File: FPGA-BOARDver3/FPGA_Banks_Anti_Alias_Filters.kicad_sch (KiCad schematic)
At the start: 10 parts, among them U1 XC7Z020-1CLG400I__

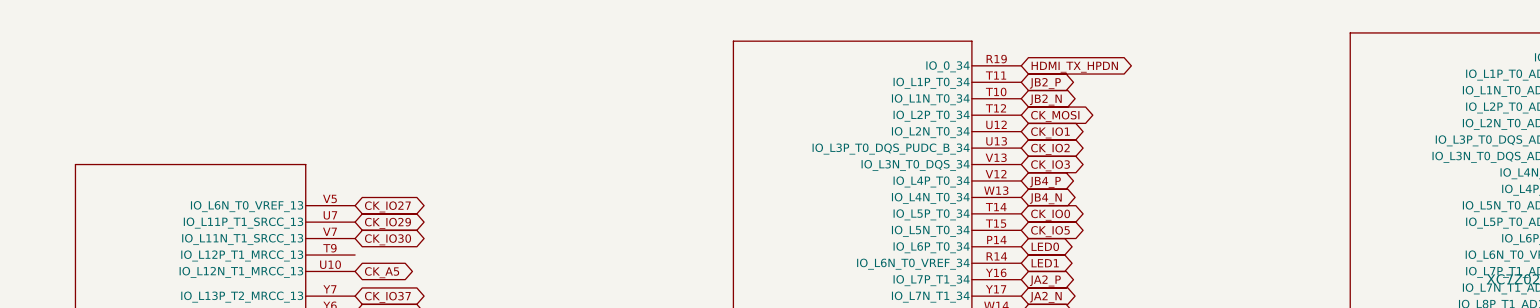
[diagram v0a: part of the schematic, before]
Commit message: update
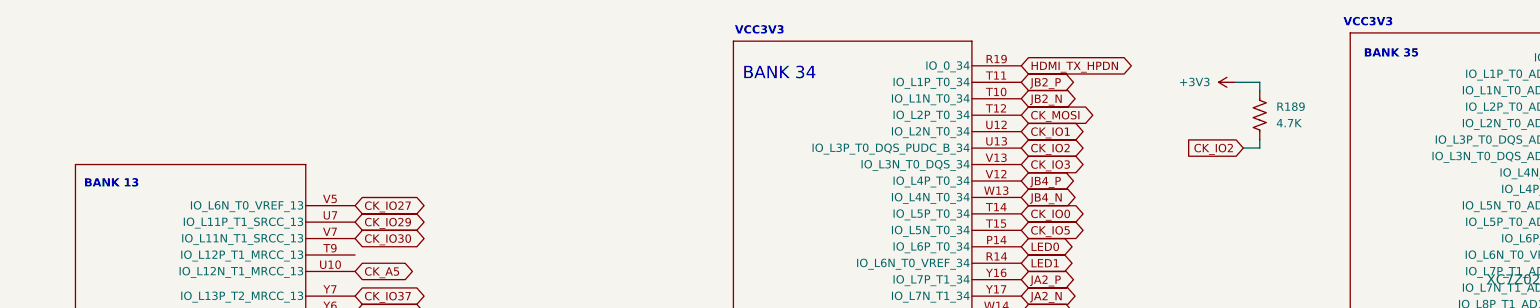
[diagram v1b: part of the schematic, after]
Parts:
- added R189: 4.7K, footprints:R_0402, symbol Device:R_US
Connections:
- net CK_IO2: now also R189.1
- new net +3V3: R189.2
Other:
- note added: "BANK 13"
- note added: "BANK 34"
- note added: "BANK 35"
- note added: "VCC3V3"

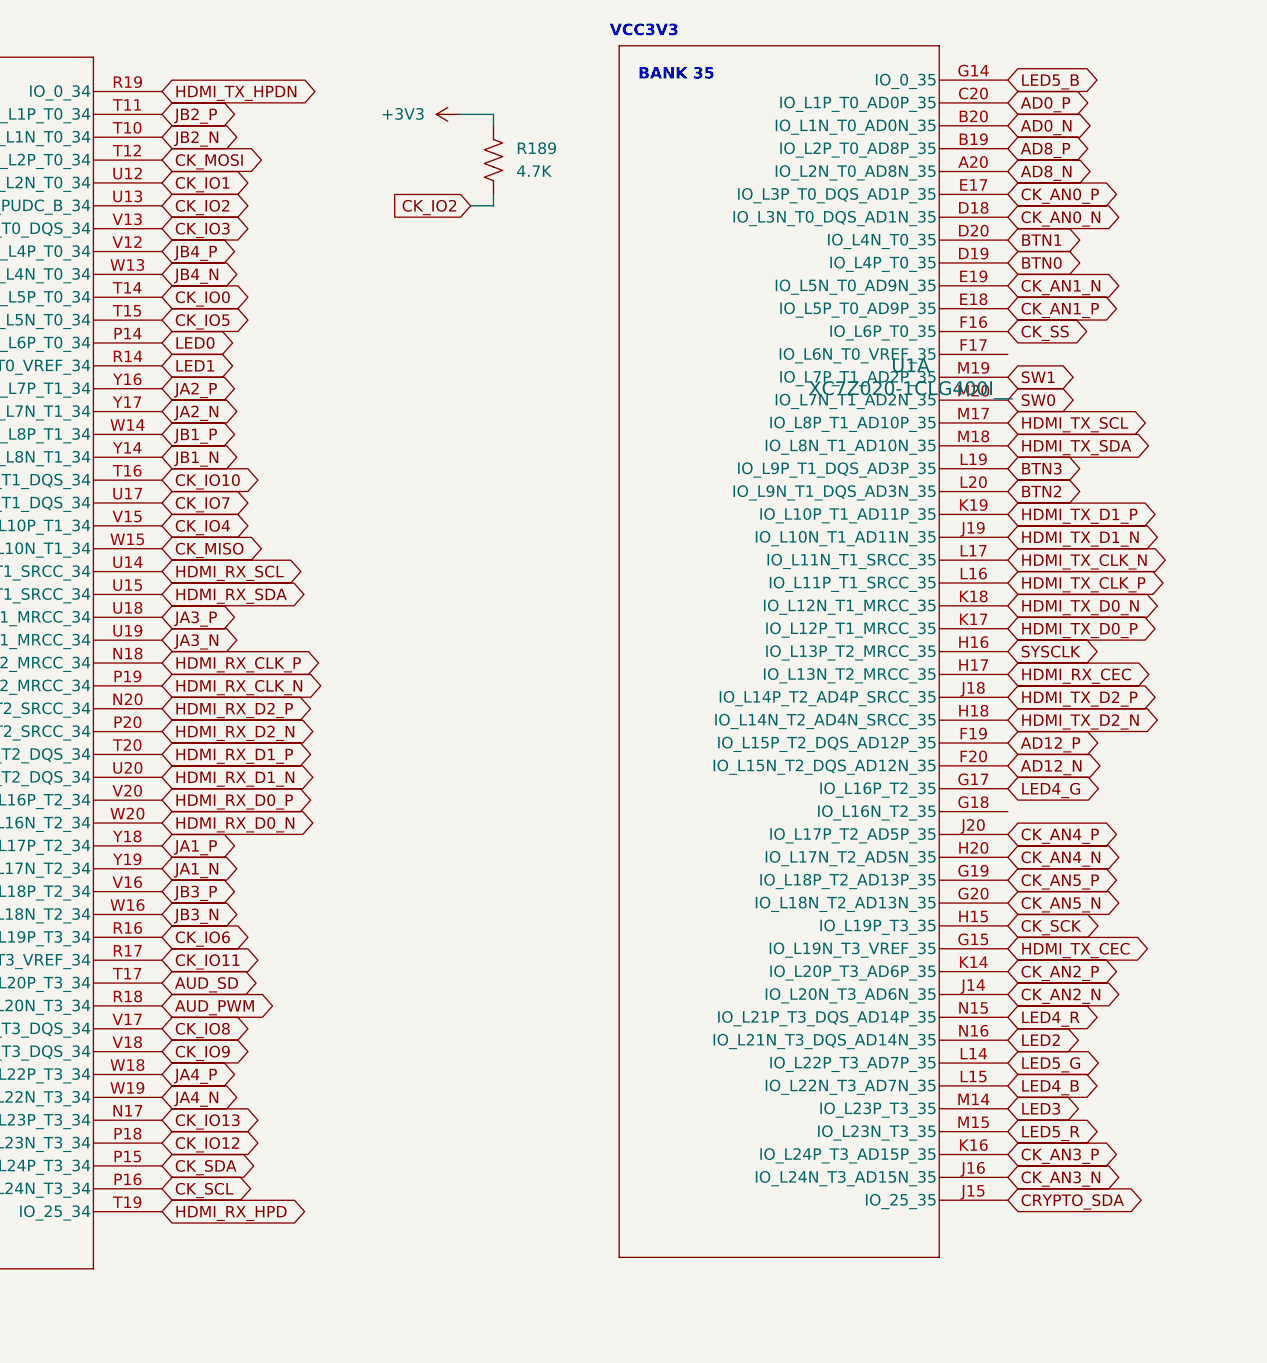
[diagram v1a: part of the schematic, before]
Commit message: schematic pages for review
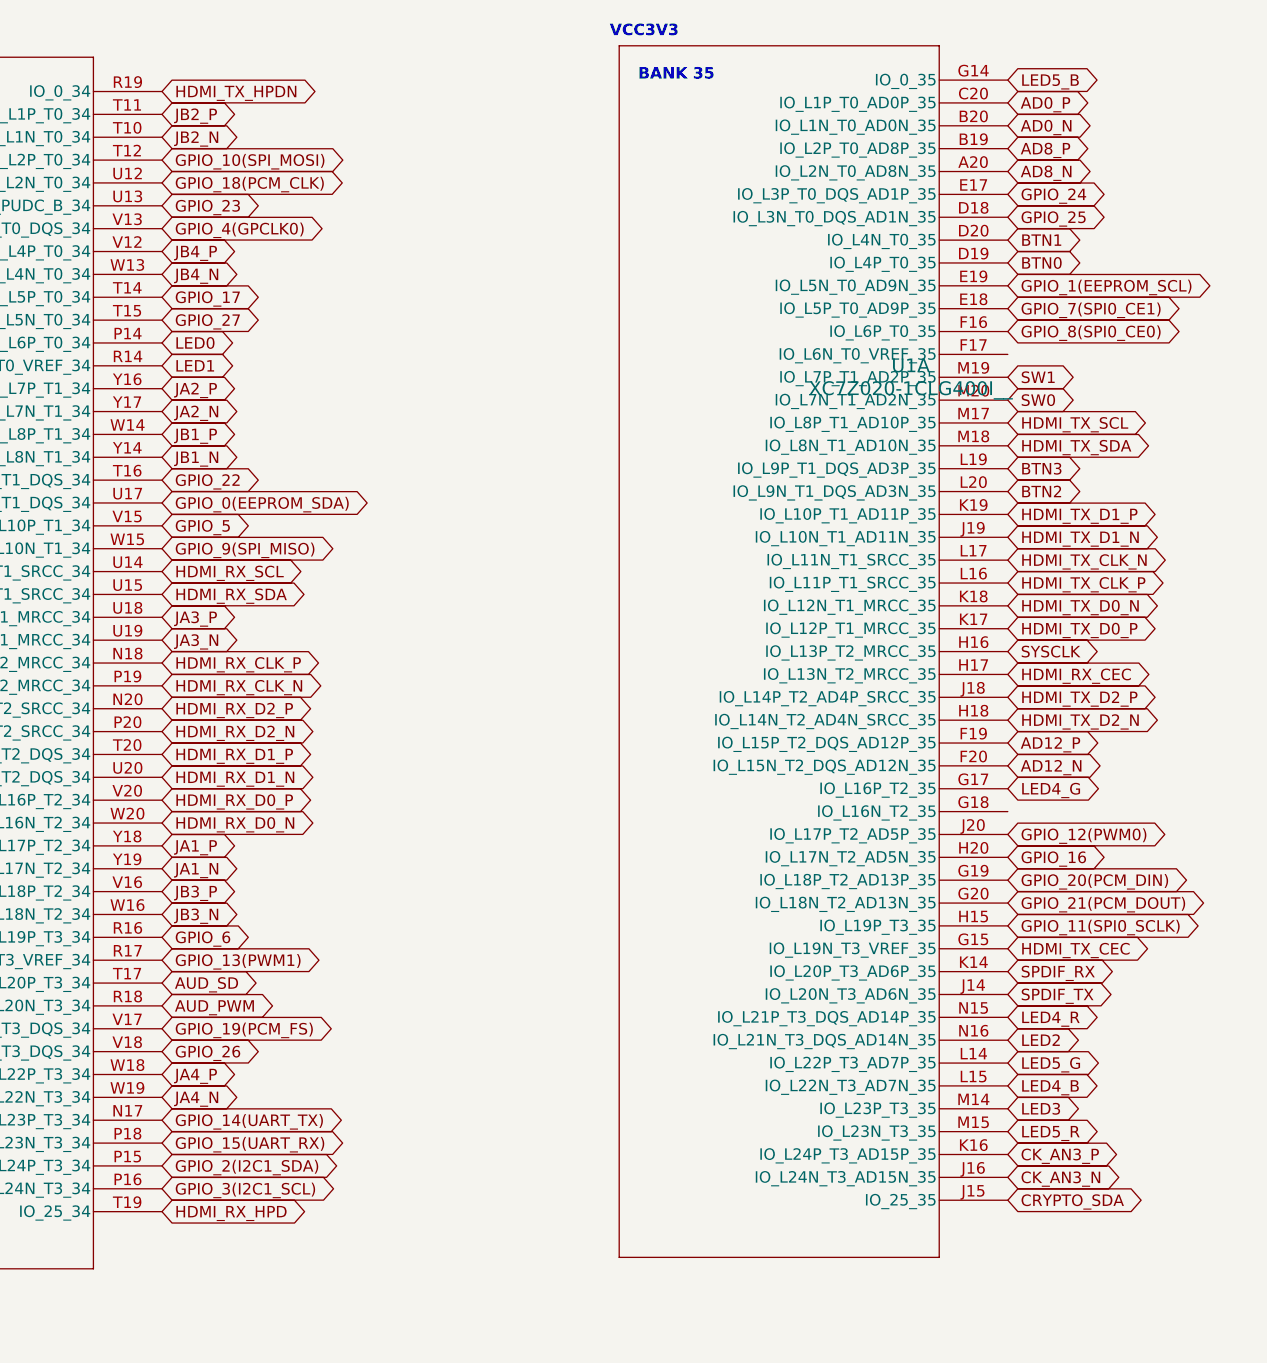
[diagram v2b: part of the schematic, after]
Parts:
- removed R189: 4.7K, footprints:R_0402, symbol Device:R_US
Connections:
- net CK_AN0_N renamed GPIO_25
- net CK_AN0_P renamed GPIO_24
- net CK_AN1_N renamed GPIO_1(EEPROM_SCL)
- net CK_AN1_P renamed GPIO_7(SPI0_CE1)
- net CK_AN2_N renamed SPDIF_TX
- net CK_AN2_P renamed SPDIF_RX
- net CK_AN4_N renamed GPIO_16
- net CK_AN4_P renamed GPIO_12(PWM0)
- net CK_AN5_N renamed GPIO_21(PCM_DOUT)
- net CK_AN5_P renamed GPIO_20(PCM_DIN)
- net CK_IO0 renamed GPIO_17
- net CK_IO1 renamed GPIO_18(PCM_CLK)
- net CK_IO10 renamed GPIO_22
- net CK_IO11 renamed GPIO_13(PWM1)
- net CK_IO12 renamed GPIO_15(UART_RX)
- net CK_IO13 renamed GPIO_14(UART_TX)
- net CK_IO2 renamed GPIO_23
- net CK_IO3 renamed GPIO_4(GPCLK0)
- net CK_IO4 renamed GPIO_5
- net CK_IO5 renamed GPIO_27
- net CK_IO6 renamed GPIO_6
- net CK_IO7 renamed GPIO_0(EEPROM_SDA)
- net CK_IO8 renamed GPIO_19(PCM_FS)
- net CK_IO9 renamed GPIO_26
- net CK_MISO renamed GPIO_9(SPI_MISO)
- net CK_MOSI renamed GPIO_10(SPI_MOSI)
- net CK_SCK renamed GPIO_11(SPI0_SCLK)
- net CK_SCL renamed GPIO_3(I2C1_SCL)
- net CK_SDA renamed GPIO_2(I2C1_SDA)
- net CK_SS renamed GPIO_8(SPI0_CE0)
